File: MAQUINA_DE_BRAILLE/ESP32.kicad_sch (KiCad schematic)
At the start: 18 parts, among them J4 USB_C_Receptacle_USB2.0_16P, J5 Screw_Terminal_01x03, J6 Screw_Terminal_01x03, J7 Screw_Terminal_01x02, Q1 IRLZ44NSTRLPBF, SW1 TS-1088-AR02016, SW2 TS-1088-AR02016, U1 ESP32-S3-WROOM-1-N16

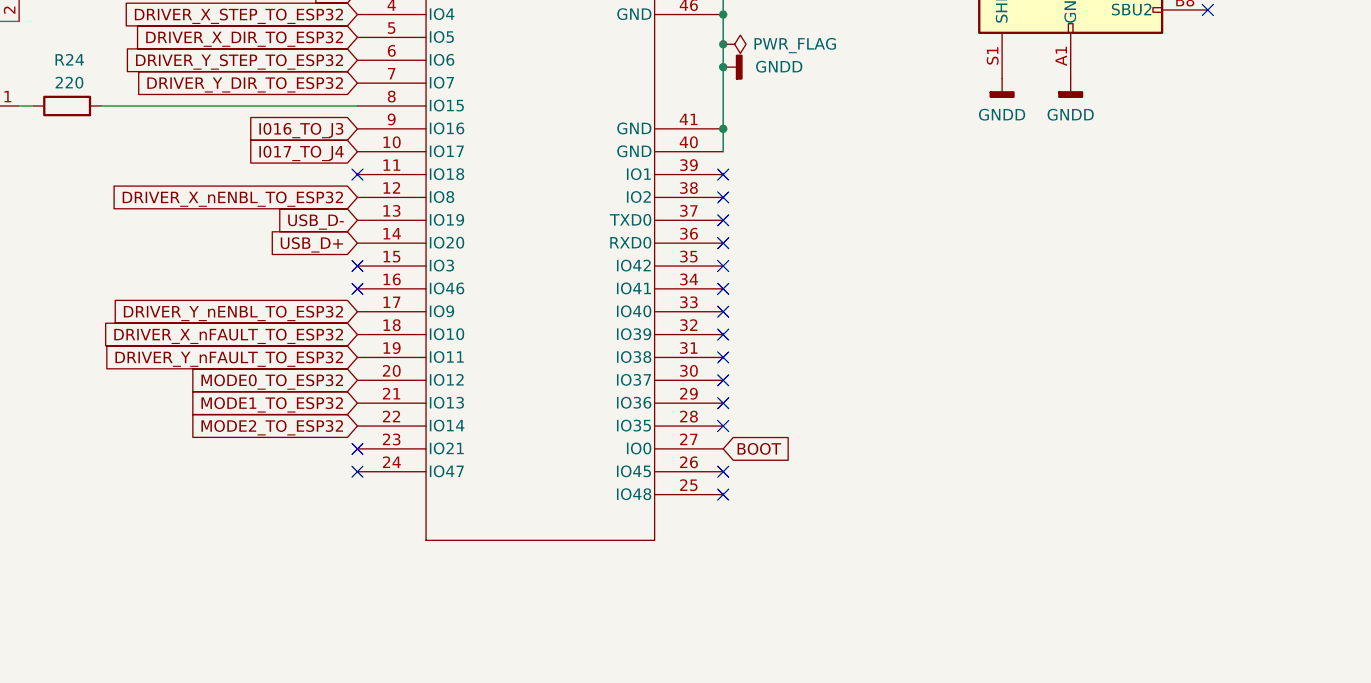
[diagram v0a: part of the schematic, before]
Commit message: tuki
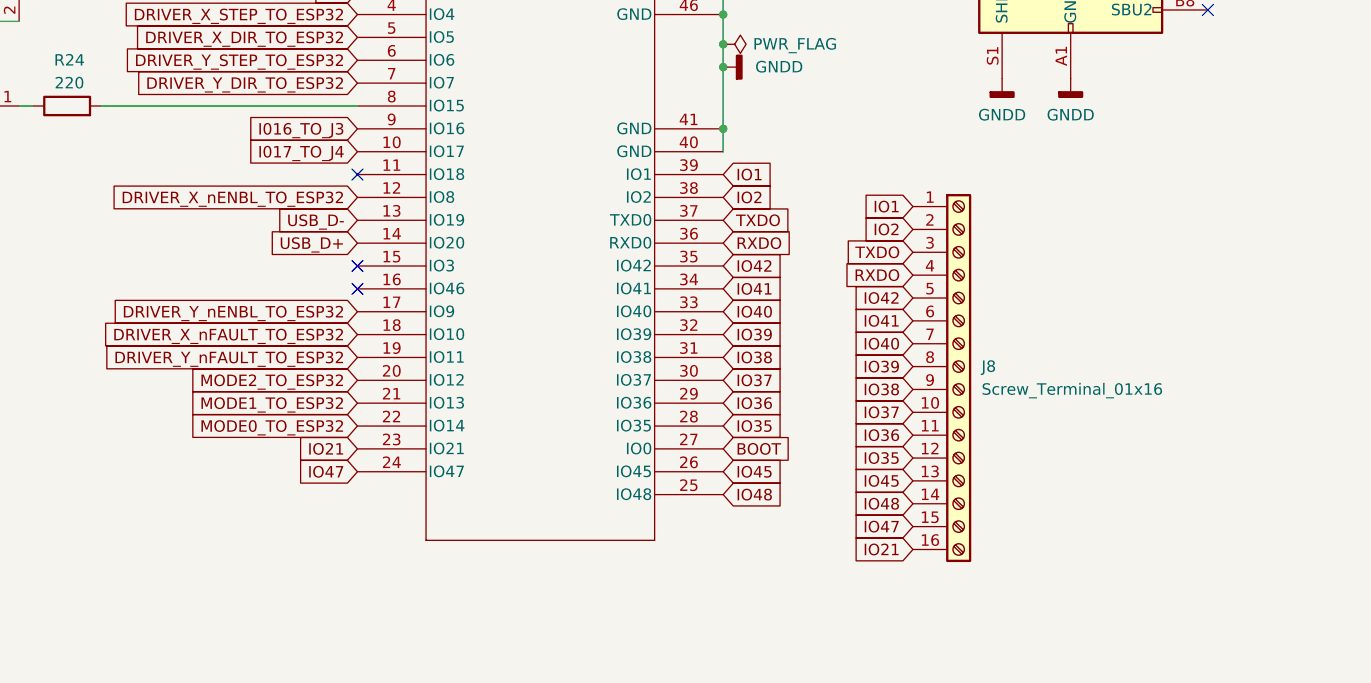
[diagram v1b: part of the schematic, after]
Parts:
- added J8: Screw_Terminal_01x16, TerminalBlock:TerminalBlock_Xinya_XY308-2.54-16P_1x16_P2.54mm_Horizontal, symbol Connector:Screw_Terminal_01x16
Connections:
- net MODE0_TO_ESP32: now also U1.22 (IO14); no longer U1.20 (IO12)
- net MODE2_TO_ESP32: now also U1.20 (IO12); no longer U1.22 (IO14)
- net IO21: now reaches U1.23 (IO21)
- net IO21: now also J8.16 (Pin_16)
- net IO47: now reaches U1.24 (IO47)
- net IO47: now also J8.15 (Pin_15)
- net IO48: now reaches U1.25 (IO48)
- net IO48: now also J8.14 (Pin_14)
- net IO45: now reaches U1.26 (IO45)
- net IO45: now also J8.13 (Pin_13)
- net IO35: now reaches U1.28 (IO35)
- net IO35: now also J8.12 (Pin_12)
- net IO36: now reaches U1.29 (IO36)
- net IO36: now also J8.11 (Pin_11)
- net IO37: now reaches U1.30 (IO37)
- net IO37: now also J8.10 (Pin_10)
- net IO38: now reaches U1.31 (IO38)
- net IO38: now also J8.9 (Pin_9)
- net IO39: now reaches U1.32 (IO39)
- net IO39: now also J8.8 (Pin_8)
- net IO40: now reaches U1.33 (IO40)
- net IO40: now also J8.7 (Pin_7)
- net IO41: now reaches U1.34 (IO41)
- net IO41: now also J8.6 (Pin_6)
- net IO42: now reaches U1.35 (IO42)
- net IO42: now also J8.5 (Pin_5)
- net RXDO: now reaches U1.36 (RXD0)
- net RXDO: now also J8.4 (Pin_4)
- net TXDO: now reaches U1.37 (TXD0)
- net TXDO: now also J8.3 (Pin_3)
- net IO2: now reaches U1.38 (IO2)
- net IO2: now also J8.2 (Pin_2)
- net IO1: now reaches U1.39 (IO1)
- net IO1: now also J8.1 (Pin_1)
- no-connect marks 21 -> 5
